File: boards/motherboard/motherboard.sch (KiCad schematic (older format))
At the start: 45 parts, among them CN1 CONN_01X02, CN2 CONN_01X02, CN3 CONN_01X02, CN4 CONN_01X02, CN5 CONN_01X02, J1 RJ45, J2 RJ45, J3 RJ45, J4 RJ45, J5 RJ45, U1 EBAYPCA9685

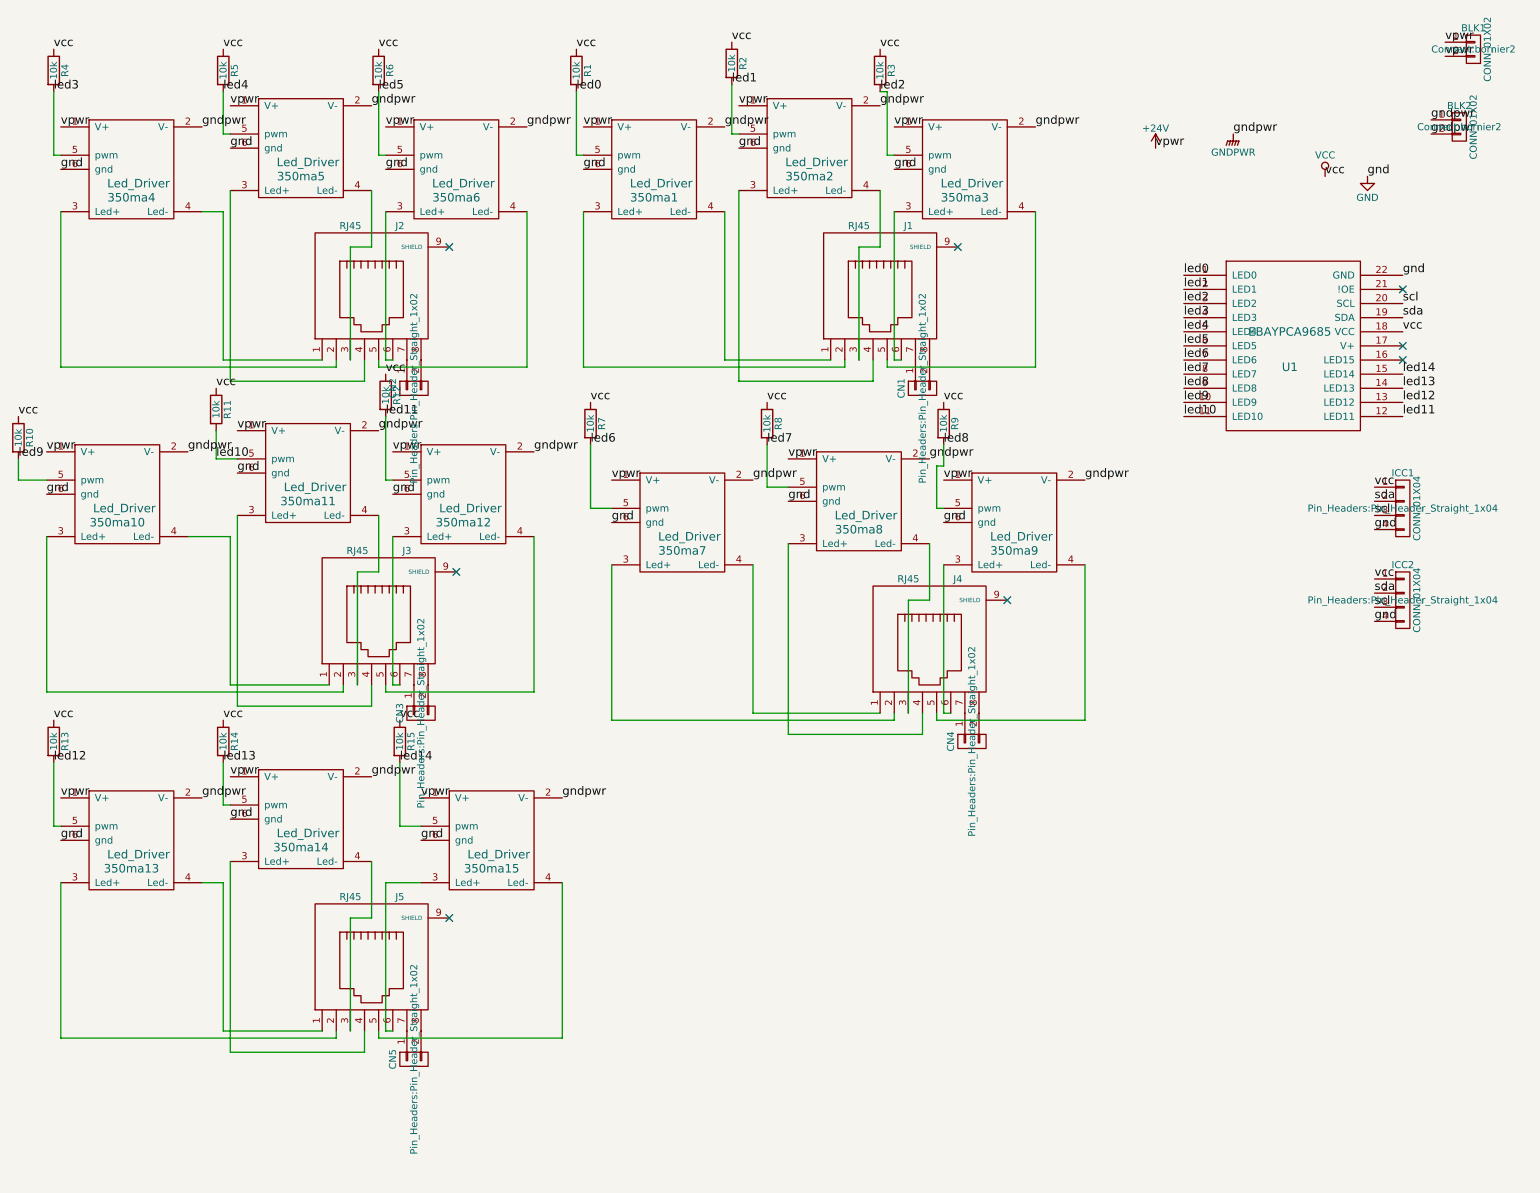
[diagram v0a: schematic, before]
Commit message: sink
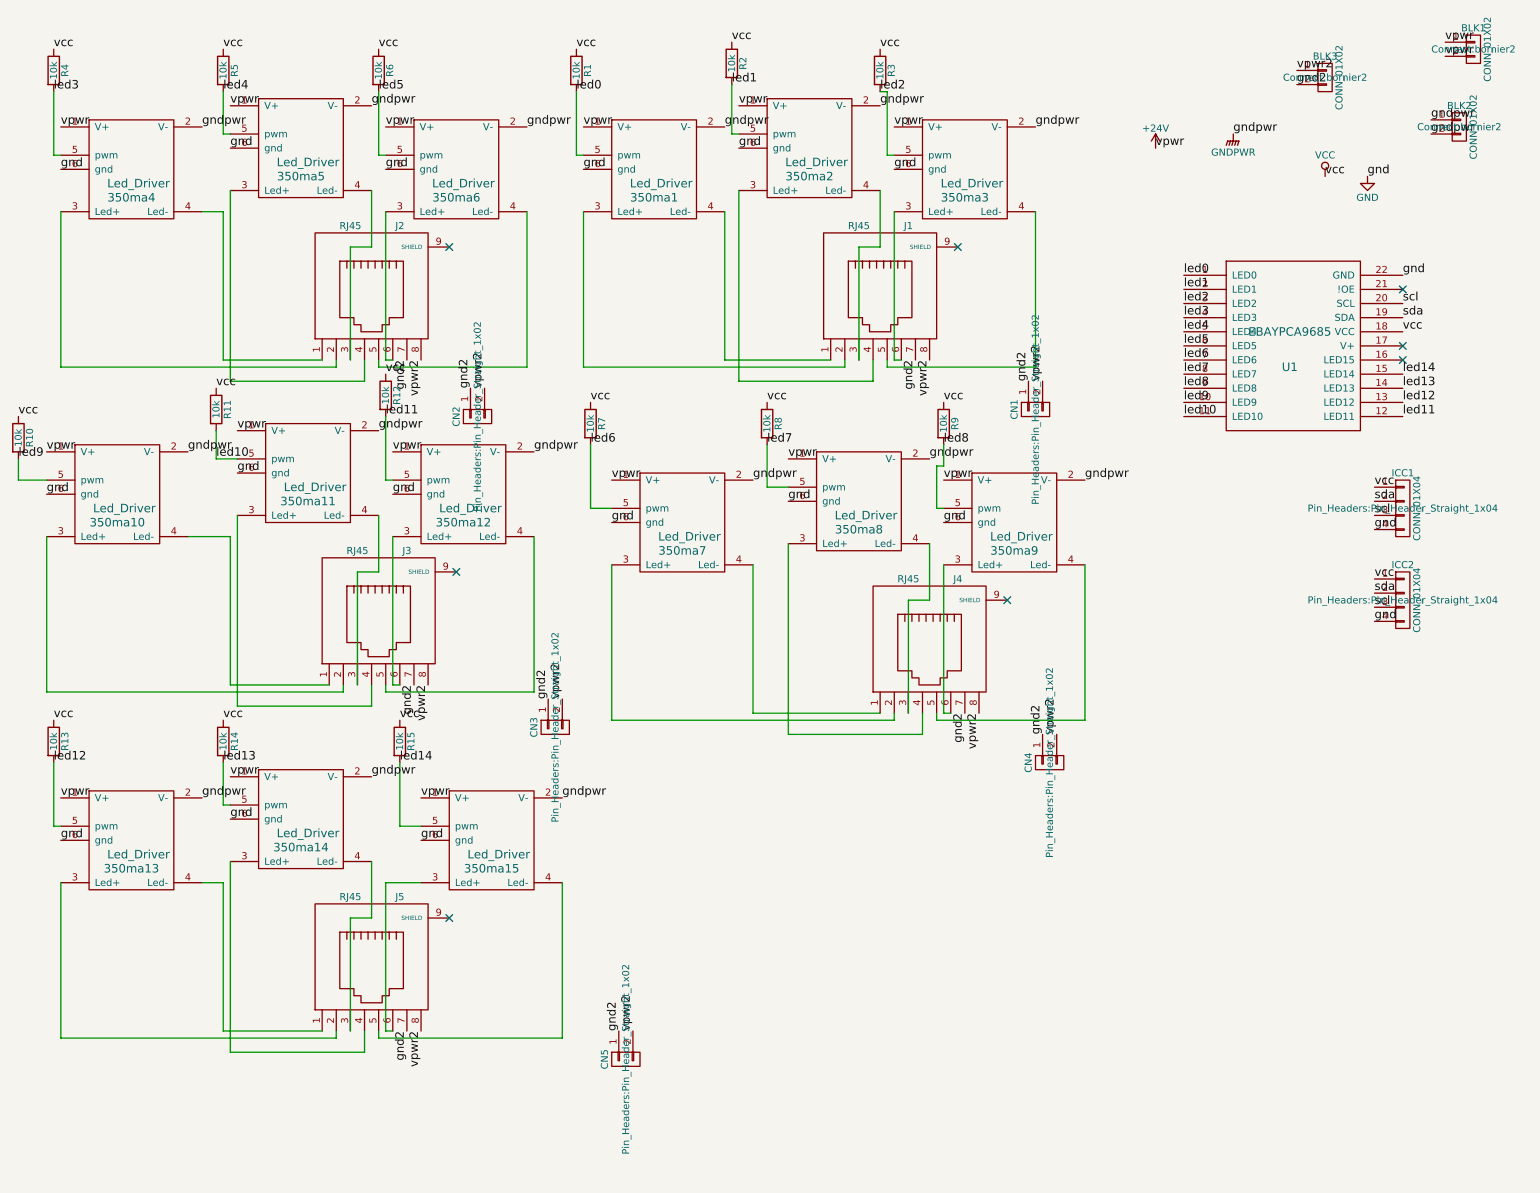
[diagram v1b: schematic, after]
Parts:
- added BLK3: CONN_01X02, Connect:bornier2, symbol CONN_01X02
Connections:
- net gnd2: now reaches CN1.1 (P1), J1.7
- net gnd2: now also CN2.1 (P1), CN3.1 (P1), CN4.1 (P1), CN5.1 (P1), J2.7, J3.7, J4.7, J5.7, BLK3.2 (P2)
- net vpwr2: now reaches CN1.2 (P2), J1.8
- net vpwr2: now also CN2.2 (P2), CN3.2 (P2), CN4.2 (P2), CN5.2 (P2), J2.8, J3.8, J4.8, J5.8, BLK3.1 (P1)
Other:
- moved on the sheet: CN1, CN2, CN3, CN4, CN5
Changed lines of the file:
@@
 L CONN_01X02 CN1
 U 1 1 5791F965
-P 6950 3050
-F 0 "CN1" H 6950 3200 50  0000 C CNN
-F 1 "CONN_01X02" V 7050 3050 50  0001 C CNN
-F 2 "Pin_Headers:Pin_Header_Straight_1x02" H 6950 3050 50  0000 C CNN
-F 3 "" H 6950 3050 50  0000 C CNN
-	1    6950 3050
+P 7750 3200
+F 0 "CN1" H 7750 3350 50  0000 C CNN
+F 1 "CONN_01X02" V 7850 3200 50  0001 C CNN
+F 2 "Pin_Headers:Pin_Header_Straight_1x02" H 7750 3200 50  0000 C CNN
+F 3 "" H 7750 3200 50  0000 C CNN
+	1    7750 3200
 	0    -1   1    0
 $EndComp
@@
 L CONN_01X02 CN2
 U 1 1 57920C53
-P 3350 3050
-F 0 "CN2" H 3350 3200 50  0000 C CNN
-F 1 "CONN_01X02" V 3450 3050 50  0001 C CNN
-F 2 "Pin_Headers:Pin_Header_Straight_1x02" H 3350 3050 50  0000 C CNN
-F 3 "" H 3350 3050 50  0000 C CNN
-	1    3350 3050
+P 3800 3250
+F 0 "CN2" H 3800 3400 50  0000 C CNN
+F 1 "CONN_01X02" V 3900 3250 50  0001 C CNN
+F 2 "Pin_Headers:Pin_Header_Straight_1x02" H 3800 3250 50  0000 C CNN
+F 3 "" H 3800 3250 50  0000 C CNN
+	1    3800 3250
 	0    -1   1    0
 $EndComp
@@
 L CONN_01X02 CN4
 U 1 1 5792107E
-P 7300 5550
-F 0 "CN4" H 7300 5700 50  0000 C CNN
-F 1 "CONN_01X02" V 7400 5550 50  0001 C CNN
-F 2 "Pin_Headers:Pin_Header_Straight_1x02" H 7300 5550 50  0000 C CNN
-F 3 "" H 7300 5550 50  0000 C CNN
-	1    7300 5550
+P 7850 5700
+F 0 "CN4" H 7850 5850 50  0000 C CNN
+F 1 "CONN_01X02" V 7950 5700 50  0001 C CNN
+F 2 "Pin_Headers:Pin_Header_Straight_1x02" H 7850 5700 50  0000 C CNN
+F 3 "" H 7850 5700 50  0000 C CNN
+	1    7850 5700
 	0    -1   1    0
 $EndComp
@@
 L CONN_01X02 CN3
 U 1 1 5792142A
-P 3400 5350
-F 0 "CN3" H 3400 5500 50  0000 C CNN
-F 1 "CONN_01X02" V 3500 5350 50  0001 C CNN
-F 2 "Pin_Headers:Pin_Header_Straight_1x02" H 3400 5350 50  0000 C CNN
-F 3 "" H 3400 5350 50  0000 C CNN
-	1    3400 5350
+P 4350 5450
+F 0 "CN3" H 4350 5600 50  0000 C CNN
+F 1 "CONN_01X02" V 4450 5450 50  0001 C CNN
+F 2 "Pin_Headers:Pin_Header_Straight_1x02" H 4350 5450 50  0000 C CNN
+F 3 "" H 4350 5450 50  0000 C CNN
+	1    4350 5450
 	0    -1   1    0
 $EndComp
@@
 L CONN_01X02 CN5
 U 1 1 579214D0
-P 3350 7800
-F 0 "CN5" H 3350 7950 50  0000 C CNN
-F 1 "CONN_01X02" V 3450 7800 50  0001 C CNN
-F 2 "Pin_Headers:Pin_Header_Straight_1x02" H 3350 7800 50  0000 C CNN
-F 3 "" H 3350 7800 50  0000 C CNN
-	1    3350 7800
+P 4850 7800
+F 0 "CN5" H 4850 7950 50  0000 C CNN
+F 1 "CONN_01X02" V 4950 7800 50  0001 C CNN
+F 2 "Pin_Headers:Pin_Header_Straight_1x02" H 4850 7800 50  0000 C CNN
+F 3 "" H 4850 7800 50  0000 C CNN
+	1    4850 7800
 	0    -1   1    0
 $EndComp
@@
 	1    0    0    -1
 $EndComp
+$Comp
+L CONN_01X02 BLK3
+U 1 1 579629B9
+P 9800 850
+F 0 "BLK3" H 9800 1000 50  0000 C CNN
+F 1 "CONN_01X02" V 9900 850 50  0000 C CNN
+F 2 "Connect:bornier2" H 9800 850 50  0000 C CNN
+F 3 "" H 9800 850 50  0000 C CNN
+	1    9800 850
+	1    0    0    -1
+$EndComp
+Text Label 9600 800  0    60   ~ 0
+vpwr2
+Text Label 9600 900  0    60   ~ 0
+gnd2
+Text Label 7800 3000 1    60   ~ 0
+vpwr2
+Text Label 7700 3000 1    60   ~ 0
+gnd2
+Text Label 6900 2850 3    60   ~ 0
+gnd2
+Text Label 7000 2850 3    60   ~ 0
+vpwr2
+Text Label 3750 3050 1    60   ~ 0
+gnd2
+Text Label 3850 3050 1    60   ~ 0
+vpwr2
+Text Label 3400 2850 3    60   ~ 0
+vpwr2
+Text Label 3300 2850 3    60   ~ 0
+gnd2
+Text Label 7900 5500 1    60   ~ 0
+vpwr2
+Text Label 4400 5250 1    60   ~ 0
+vpwr2
+Text Label 7800 5500 1    60   ~ 0
+gnd2
+Text Label 4300 5250 1    60   ~ 0
+gnd2
+Text Label 3450 5150 3    60   ~ 0
+vpwr2
+Text Label 3350 5150 3    60   ~ 0
+gnd2
+Text Label 7250 5350 3    60   ~ 0
+gnd2
+Text Label 7350 5350 3    60   ~ 0
+vpwr2
+Text Label 4800 7600 1    60   ~ 0
+gnd2
+Text Label 4900 7600 1    60   ~ 0
+vpwr2
+Text Label 3400 7600 3    60   ~ 0
+vpwr2
+Text Label 3300 7600 3    60   ~ 0
+gnd2
 $EndSCHEMATC
